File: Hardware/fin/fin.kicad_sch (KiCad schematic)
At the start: 46 parts, among them J1 Conn_01x10_Pin, J2 Conn_01x04_Pin, J3 Conn_01x04_Pin, J5 Conn_01x04_Pin, U1 ADS131M03QPWRQ1, U2 ADXL380-1BCCZ-RL7, U3 W25N512GVEIG, U4 TMP235A4DBZR, U5 STM32L412K8Ux, U6 ADXL380-1BCCZ-RL7, X1 ECS-327TXO-33-TR

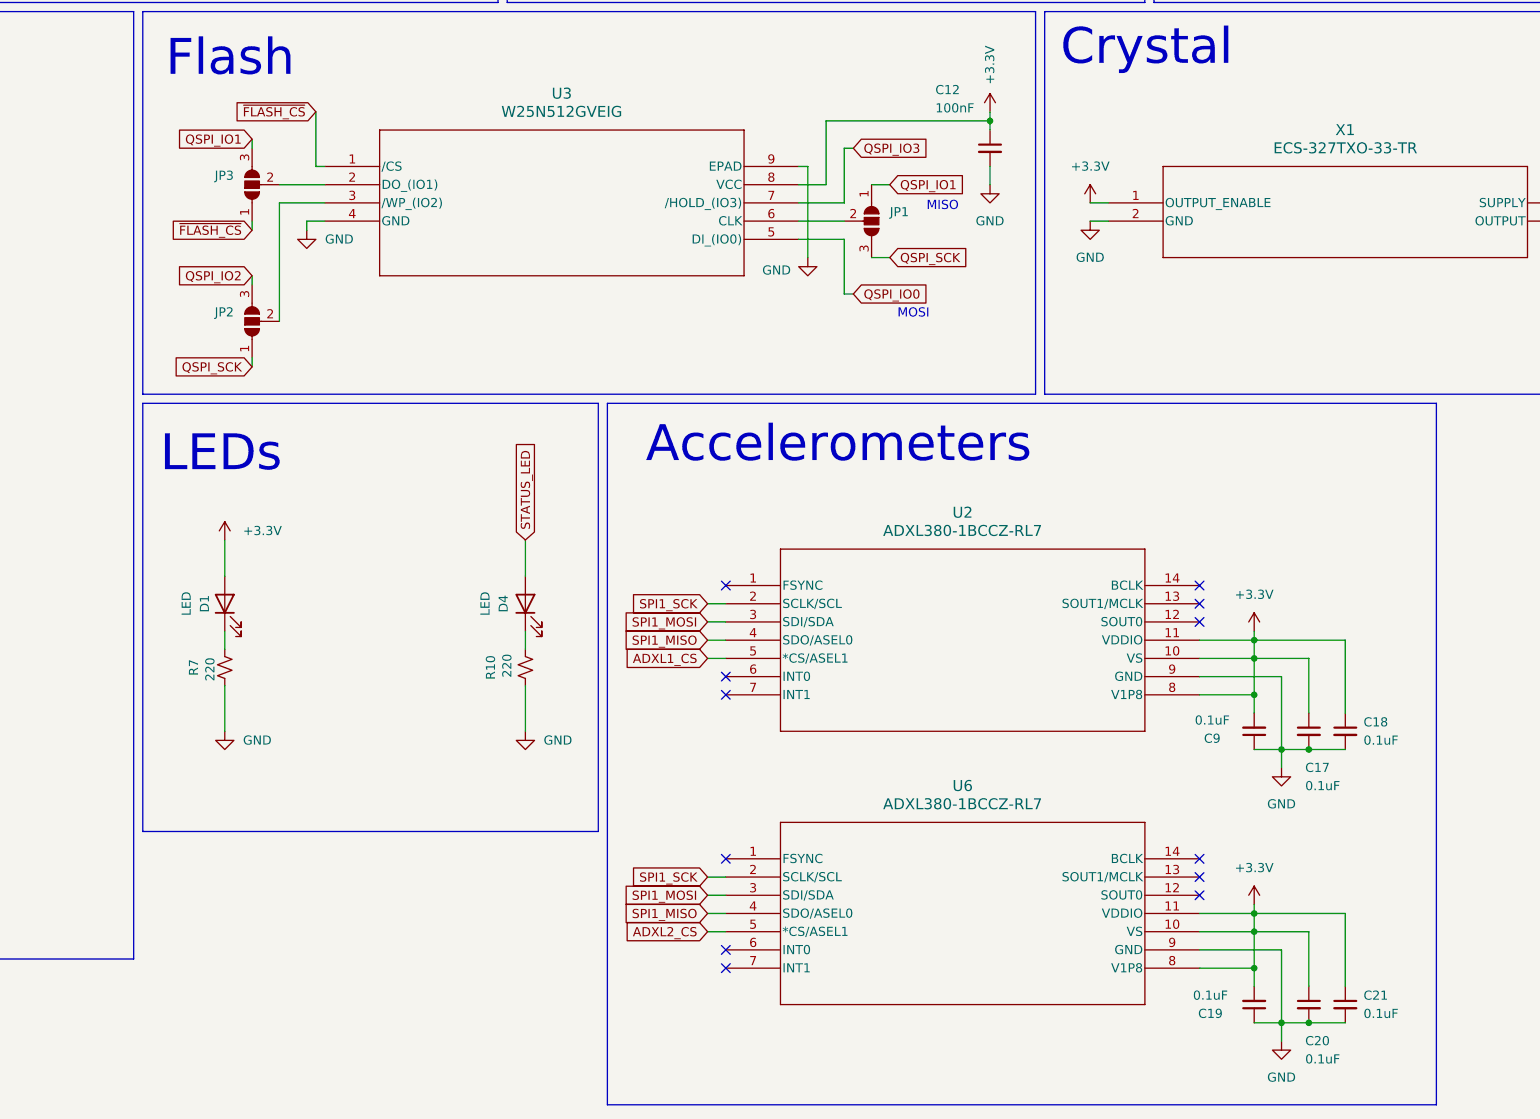
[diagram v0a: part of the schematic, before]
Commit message: oooooooooo we're half way theeerree
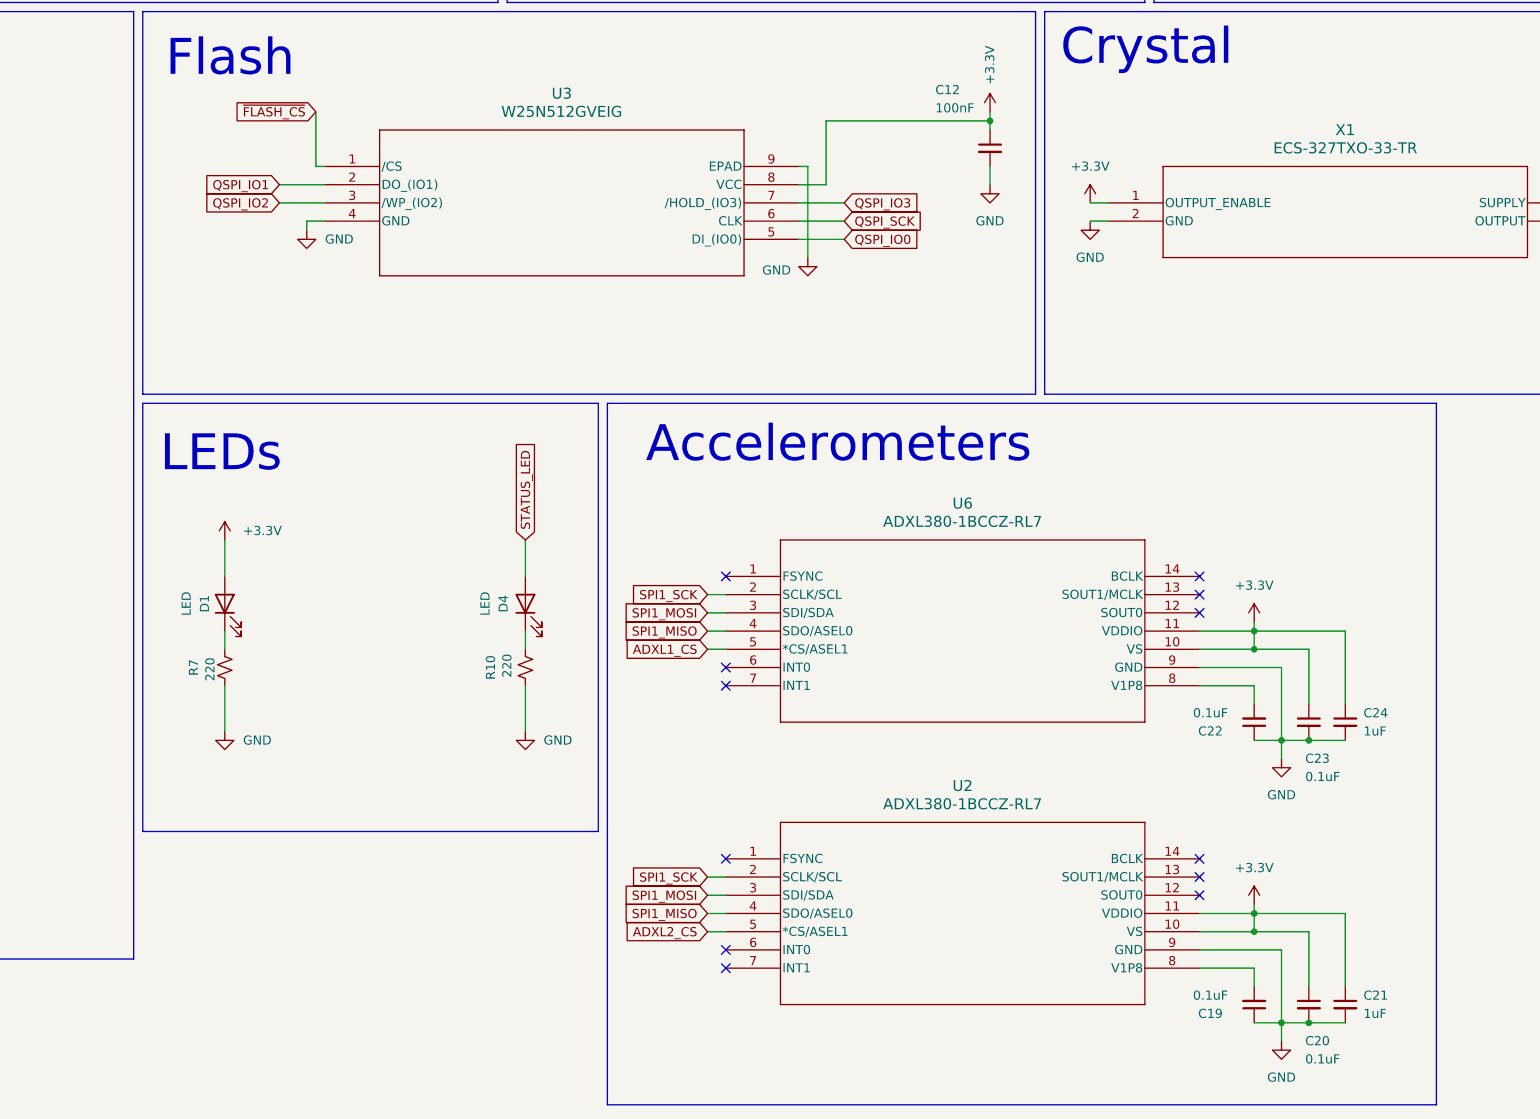
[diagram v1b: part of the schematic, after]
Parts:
- removed C17, C18, C9: 0.1uF, Capacitor_SMD:C_0603_1608Metric, symbol Device:C_Small
- removed JP1, JP2, JP3: SolderJumper_3_Open, Jumper:SolderJumper-3_P1.3mm_Open_RoundedPad1.0x1.5mm, symbol Jumper:SolderJumper_3_Open
- added C22, C23: 0.1uF, Capacitor_SMD:C_0402_1005Metric, symbol Device:C_Small
- added C24: 1uF, Capacitor_SMD:C_0402_1005Metric, symbol Device:C_Small
- C1, C10, C11, C12, C13, C14, C15, C16, C19, C2, C20, C3, C4, C5: footprint Capacitor_SMD:C_0603_1608Metric -> Capacitor_SMD:C_0402_1005Metric
- C21: value 0.1uF -> 1uF; footprint Capacitor_SMD:C_0603_1608Metric -> Capacitor_SMD:C_0402_1005Metric
- D1, D4: footprint LED_SMD:LED_0603_1608Metric -> LED_SMD:LED_0402_1005Metric
- R1, R10, R11, R12, R13, R14, R2, R3, R4, R5, R6, R7: footprint Resistor_SMD:R_0603_1608Metric -> Resistor_SMD:R_0402_1005Metric
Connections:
- net +3.3V: now also C23.1, C24.1; no longer C19.2, U2.8 (V1P8), U6.8 (V1P8)
- net ADXL1_CS: now also U6.5 (*CS/ASEL1); no longer U2.5 (*CS/ASEL1)
- net ADXL2_CS: now also U2.5 (*CS/ASEL1); no longer U6.5 (*CS/ASEL1)
- net GND: now also C22.1, C23.2, C24.2
- net QSPI_IO1: now also U3.2 (DO_(IO1))
- net QSPI_IO2: now also U3.3 (/WP_(IO2))
- net QSPI_SCK: now also U3.6 (CLK)
- new net: C22.2, U6.8 (V1P8)
- new net: C19.2, U2.8 (V1P8)
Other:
- note removed: "MISO"
- note removed: "MOSI"
